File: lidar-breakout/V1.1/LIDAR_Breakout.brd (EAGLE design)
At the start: 36.5 x 88 mm, 89 parts, among them J1 UX60-MB-5S8, J2 AVR_SPI_PROG_3X2TESTPOINTS, P1 MOLEX 0436500200, X1 TSX-3225 16.0000MF18X-AC0

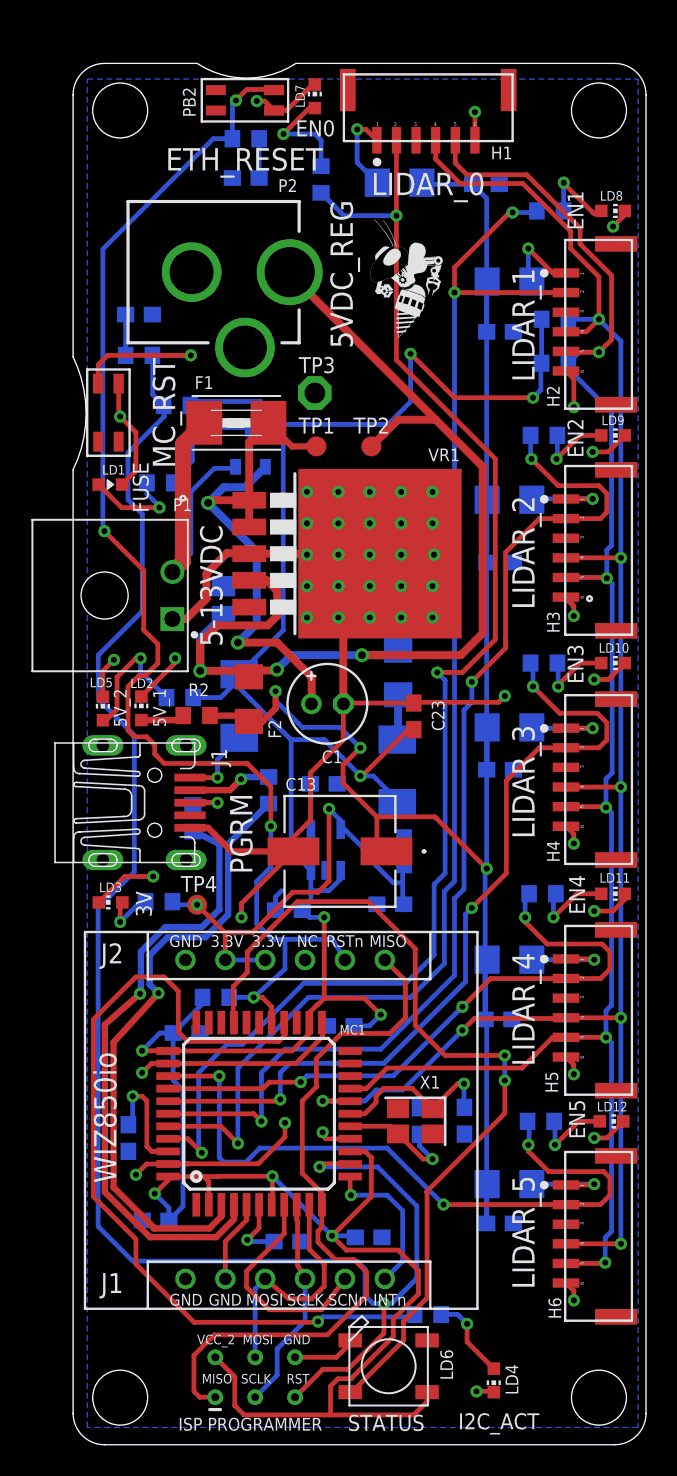
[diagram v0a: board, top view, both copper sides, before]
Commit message: Updated Reset PB
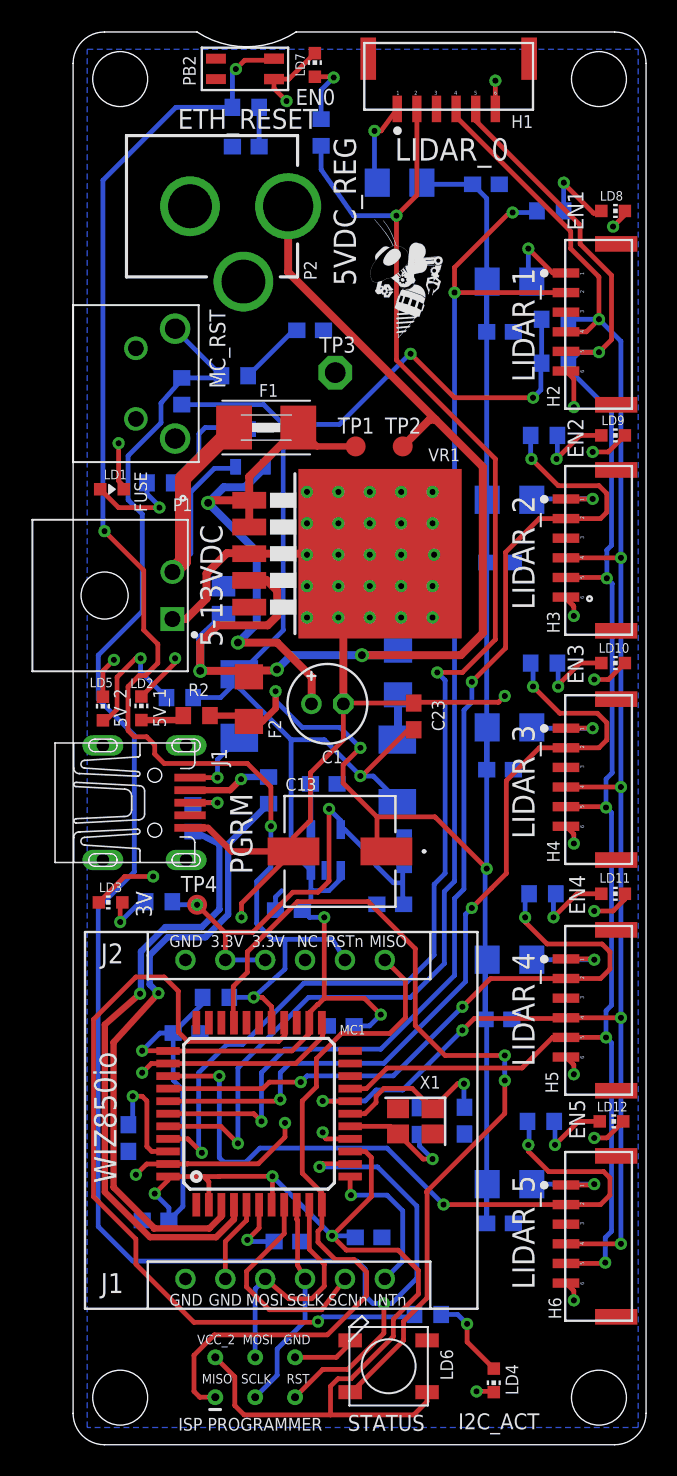
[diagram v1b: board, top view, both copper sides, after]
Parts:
- PB1: device RoboJackets-Switches:RESET_PB_RA -> RoboJackets-Switches:TACT_PB_RA
- moved C26 10.9 mm to (15.1, 71.0)
- moved R19 6.24 mm to (10.3, 68.1), turned to 180 degrees
- moved P2 4.20 mm to (0.10, 78.9)
- moved PB1 4.20 mm to (0.00, 72.6)
- moved R7 3.00 mm to (15.8, 83.6)
- moved TP1 2.50 mm to (18.0, 63.6)
- moved H1 2.39 mm to (29.3, 89.3)
- moved C25 2.00 mm to (11.0, 82.7)
- moved LD7 2.00 mm to (15.4, 87.9)
- moved PB2 2.00 mm to (13.7, 89.0)
- moved R18 2.00 mm to (11.0, 85.2)
- moved TP2 2.00 mm to (21.0, 63.6)
- moved F1 1.92 mm to (12.3, 64.8)
- moved TP3 1.84 mm to (16.7, 68.3)
- moved R1 0.95 mm to (6.92, 67.1), turned to 90 degrees
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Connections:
- net GND: now also PB1.P$2; no longer PB1.P$3
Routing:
- net LDR0_EN: track 88.7 -> 93.7 mm
- net RST_MC: track 117.1 -> 112.7 mm, vias 3 -> 2
- net GND: track 138.4 -> 134.7 mm
- net RST_ETH: track 84.9 -> 88.3 mm
- net LDR0_LED: track 6.90 -> 4.20 mm
- net 5VREG: track 69.9 -> 72.2 mm
- net N$11: track 2.60 -> 4.30 mm
- net VCC_2: track 194.9 -> 193.5 mm
- net VIN: track 36.1 -> 37.1 mm
- net SCL: track 115.4 -> 114.5 mm
- net SDA: track 109.9 -> 109.1 mm
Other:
- board size 36.5 x 88 mm -> 36.5 x 90 mm
